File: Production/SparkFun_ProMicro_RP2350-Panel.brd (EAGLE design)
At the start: 92.7 x 87.1 mm, 702 parts, among them J1 QWIIC_RIGHT_ANGLE, J12 USB Female Type C Connector, J13 QWIIC_RIGHT_ANGLE, J16 USB Female Type C Connector, J17 QWIIC_RIGHT_ANGLE, J2 QWIIC_RIGHT_ANGLE, J20 USB Female Type C Connector, J21 QWIIC_RIGHT_ANGLE, J24 USB Female Type C Connector, J5 USB Female Type C Connector, J8 USB Female Type C Connector, J9 QWIIC_RIGHT_ANGLE, U1 RT9080-33GJ5, U10 W25QXX128MBIT, U11 WS2812_2020, U12 RP2350A, U13 RT9080-33GJ5, U14 W25QXX128MBIT, U15 WS2812_2020, U16 RP2350A, U17 RT9080-33GJ5, U18 W25QXX128MBIT, U19 WS2812_2020, U2 RP2350A, U20 RP2350A, U21 RT9080-33GJ5, U22 W25QXX128MBIT, U23 WS2812_2020, U24 RP2350A, U3 WS2812_2020, U4 W25QXX128MBIT, U5 RT9080-33GJ5, U6 W25QXX128MBIT, U7 WS2812_2020, U8 RP2350A, U9 RT9080-33GJ5, Y1 12MHz, Y2 12MHz, Y3 12MHz, Y4 12MHz, Y5 12MHz, Y6 12MHz

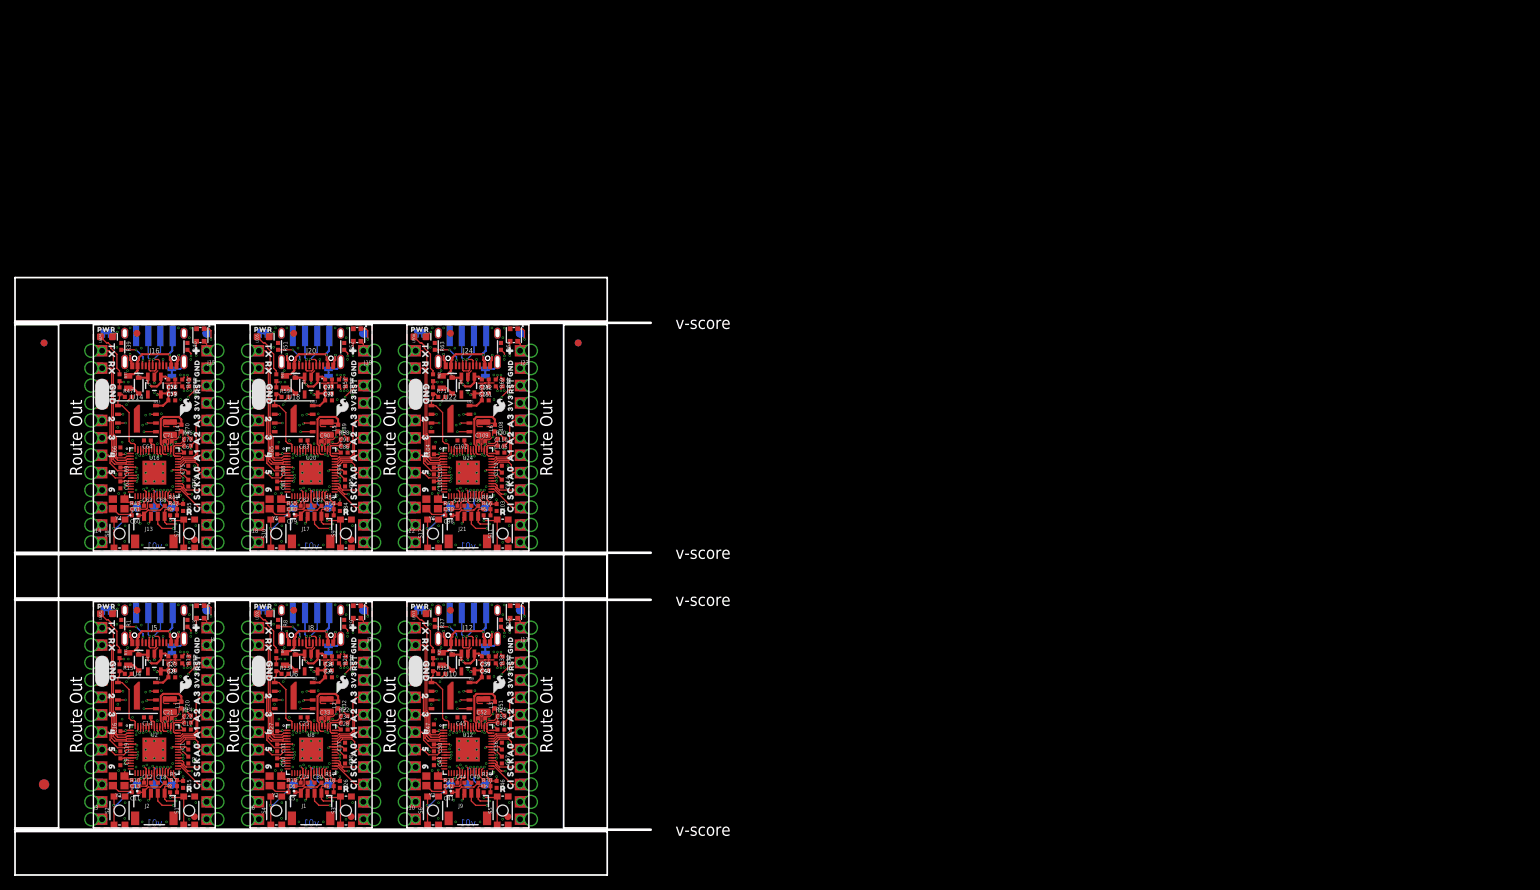
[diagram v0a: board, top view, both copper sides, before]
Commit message: Add v10 production files
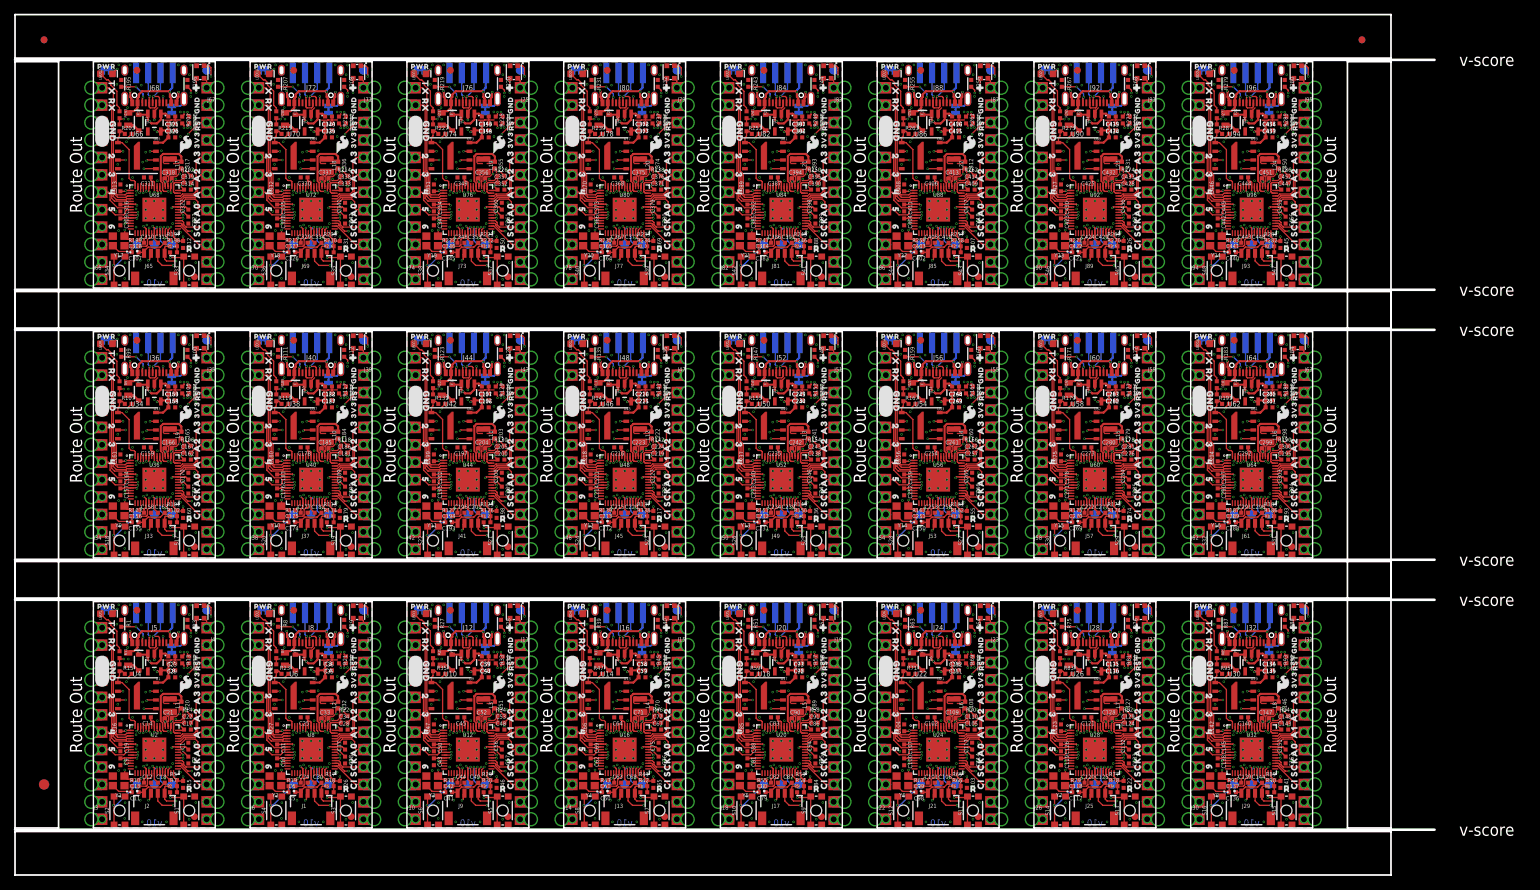
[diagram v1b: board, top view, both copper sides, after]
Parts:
- added C115, C116, C127, C128, C134, C135, C146, C147, C153, C154, C165, C166, C172, C173, C184, C185, C191, C192, C203, C204, C210, C211, C222, C223, C229, C230, C241, C242, C248, C249, C260, C261, C267, C268, C279, C280, C286, C287, C298, C299, C305, C306, C317, C318, C324, C325, C336, C337, C343, C344, C355, C356, C362, C363, C374, C375, C381, C382, C393, C394, C400, C401, C412, C413, C419, C420, C431, C432, C438, C439, C450, C451: 10uF, SparkFun-Capacitors:0402-TIGHT
- added C117, C118, C136, C137, C155, C156, C174, C175, C193, C194, C212, C213, C231, C232, C250, C251, C269, C270, C288, C289, C307, C308, C326, C327, C345, C346, C364, C365, C383, C384, C402, C403, C421, C422, C440, C441: 15pF, SparkFun-Capacitors:0402-TIGHT
- added C119, C120, C121, C122, C123, C124, C125, C126, C130, C132, C133, C138, C139, C140, C141, C142, C143, C144, C145, C149, C151, C152, C157, C158, C159, C160, C161, C162, C163, C164, C168, C170, C171, C176, C177, C178, C179, C180, C181, C182, C183, C187, C189, C190, C195, C196, C197, C198, C199, C200, C201, C202, C206, C208, C209, C214, C215, C216, C217, C218, C219, C220, C221, C225, C227, C228, C233, C234, C235, C236, C237, C238, C239, C240, C244, C246, C247, C252, C253, C254, C255, C256, C257, C258, C259, C263, C265, C266, C271, C272, C273, C274, C275, C276, C277, C278, C282, C284, C285, C290, C291, C292, C293, C294, C295, C296, C297, C301, C303, C304, C309, C310, C311, C312, C313, C314, C315, C316, C320, C322, C323, C328, C329, C330, C331, C332, C333, C334, C335, C339, C341, C342, C347, C348, C349, C350, C351, C352, C353, C354, C358, C360, C361, C366, C367, C368, C369, C370, C371, C372, C373, C377, C379, C380, C385, C386, C387, C388, C389, C390, C391, C392, C396, C398, C399, C404, C405, C406, C407, C408, C409, C410, C411, C415, C417, C418, C423, C424, C425, C426, C427, C428, C429, C430, C434, C436, C437, C442, C443, C444, C445, C446, C447, C448, C449, C453, C455, C456: 0.1uF, SparkFun-Capacitors:0402-TIGHT
- added C129, C131, C148, C150, C167, C169, C186, C188, C205, C207, C224, C226, C243, C245, C262, C264, C281, C283, C300, C302, C319, C321, C338, C340, C357, C359, C376, C378, C395, C397, C414, C416, C433, C435, C452, C454: 2.2uF, SparkFun-Capacitors:0402-TIGHT
- added D10, D11, D12, D13, D14, D15, D16, D17, D18, D19, D20, D21, D22, D23, D24, D7, D8, D9: 3A/10V/280mV, SparkFun-DiscreteSemi:SOD-323
- added F10, F11, F12, F13, F14, F15, F16, F17, F18, F19, F20, F21, F22, F23, F24, F7, F8, F9: 6V 0.5A, SparkFun-Fuses:0805
- added J25, J29, J33, J37, J41, J45, J49, J53, J57, J61, J65, J69, J73, J77, J81, J85, J89, J93: QWIIC_RIGHT_ANGLE, SparkFun-Connectors:JST04_1MM_RA
- added J26, J27, J30, J31, J34, J35, J38, J39, J42, J43, J46, J47, J50, J51, J54, J55, J58, J59, J62, J63, J66, J67, J70, J71, J74, J75, J78, J79, J82, J83, J86, J87, J90, J91, J94, J95: (no value), SparkFun-Connectors:1X12_CASTELLATED
- added J28, J32, J36, J40, J44, J48, J52, J56, J60, J64, J68, J72, J76, J80, J84, J88, J92, J96: USB Female Type C Connector, SparkFun-Connectors:USB-C-16P_4LAYER-PADS
- added JP19, JP20, JP22, JP23, JP25, JP26, JP28, JP29, JP31, JP32, JP34, JP35, JP37, JP38, JP40, JP41, JP43, JP44, JP46, JP47, JP49, JP50, JP52, JP53, JP55, JP56, JP58, JP59, JP61, JP62, JP64, JP65, JP67, JP68, JP70, JP71: FIDUCIAL1X2, SparkFun-Aesthetics:FIDUCIAL-1X2
- added JP21, JP24, JP27, JP30, JP33, JP36, JP39, JP42, JP45, JP48, JP51, JP54, JP57, JP60, JP63, JP66, JP69, JP72: USB_SOLDER_PADS, SparkFun-Connectors:USB-SOLDER-PADS
- added L10, L11, L12, L13, L14, L15, L16, L17, L18, L19, L20, L21, L22, L23, L24, L7, L8, L9: 4.7μH, SparkFun-Coils:1008(2520)
- added LED10, LED11, LED12, LED13, LED14, LED15, LED16, LED17, LED18, LED19, LED20, LED21, LED22, LED23, LED24, LED7, LED8, LED9: Red, SparkFun-LED:LED-0603
- added LOGO19, LOGO22, LOGO25, LOGO28, LOGO31, LOGO34, LOGO37, LOGO40, LOGO43, LOGO46, LOGO49, LOGO52, LOGO55, LOGO58, LOGO61, LOGO64, LOGO67, LOGO70: SFE_LOGO_NAME_FLAME.1_INCH, SparkFun-Aesthetics:SFE_LOGO_NAME_FLAME_.1
- added LOGO20, LOGO23, LOGO26, LOGO29, LOGO32, LOGO35, LOGO38, LOGO41, LOGO44, LOGO47, LOGO50, LOGO53, LOGO56, LOGO59, LOGO62, LOGO65, LOGO68, LOGO71: QWIIC_LOGO_6MM, SparkFun-Aesthetics:QWIIC_6MM
- added LOGO21, LOGO24, LOGO27, LOGO30, LOGO33, LOGO36, LOGO39, LOGO42, LOGO45, LOGO48, LOGO51, LOGO54, LOGO57, LOGO60, LOGO63, LOGO66, LOGO69, LOGO72: SFE_LOGO_FLAME.1_INCH, SparkFun-Aesthetics:SFE_LOGO_FLAME_.1
- added PWR10, PWR11, PWR12, PWR13, PWR14, PWR15, PWR16, PWR17, PWR18, PWR19, PWR20, PWR21, PWR22, PWR23, PWR6, PWR7, PWR8, PWR9, SHLD10, SHLD11, SHLD12, SHLD13, SHLD14, SHLD15, SHLD16, SHLD17, SHLD18, SHLD19, SHLD20, SHLD21, SHLD22, SHLD23, SHLD6, SHLD7, SHLD8, SHLD9: JUMPER-SMT_2_NC_TRACE_SILK, SparkFun-Jumpers:SMT-JUMPER_2_NC_TRACE_SILK
- added R100, R111, R112, R123, R124, R135, R136, R147, R148, R159, R160, R171, R172, R183, R184, R195, R196, R207, R208, R219, R220, R231, R232, R243, R244, R255, R256, R267, R268, R279, R280, R75, R76, R87, R88, R99: 5.1k, SparkFun-Resistors:0402-TIGHT
- added R101, R102, R113, R114, R125, R126, R137, R138, R149, R150, R161, R162, R173, R174, R185, R186, R197, R198, R209, R210, R221, R222, R233, R234, R245, R246, R257, R258, R269, R270, R281, R282, R77, R78, R89, R90: 2.2k, SparkFun-Resistors:0402-TIGHT
- added R103, R107, R115, R119, R127, R131, R139, R143, R151, R155, R163, R167, R175, R179, R187, R191, R199, R203, R211, R215, R223, R227, R235, R239, R247, R251, R259, R263, R271, R275, R283, R287, R79, R83, R91, R95: 1k, SparkFun-Resistors:0402-TIGHT
- added R104, R105, R116, R117, R128, R129, R140, R141, R152, R153, R164, R165, R176, R177, R188, R189, R200, R201, R212, R213, R224, R225, R236, R237, R248, R249, R260, R261, R272, R273, R284, R285, R80, R81, R92, R93: 27, SparkFun-Resistors:0402-TIGHT
- added R106, R118, R130, R142, R154, R166, R178, R190, R202, R214, R226, R238, R250, R262, R274, R286, R82, R94: 10Ω, SparkFun-Resistors:0402-TIGHT
- added R108, R110, R120, R122, R132, R134, R144, R146, R156, R158, R168, R170, R180, R182, R192, R194, R204, R206, R216, R218, R228, R230, R240, R242, R252, R254, R264, R266, R276, R278, R288, R74, R84, R86, R96, R98: 10k, SparkFun-Resistors:0402-TIGHT
- added R109, R121, R133, R145, R157, R169, R181, R193, R205, R217, R229, R241, R253, R265, R277, R73, R85, R97: 4.7k, SparkFun-Resistors:0402-TIGHT
- added S13, S15, S17, S19, S21, S23, S25, S27, S29, S31, S33, S35, S37, S39, S41, S43, S45, S47: Reset, SparkFun-Switches:TACTILE_SWITCH_SMD_4.6X2.8MM
- added S14, S16, S18, S20, S22, S24, S26, S28, S30, S32, S34, S36, S38, S40, S42, S44, S46, S48: Boot, SparkFun-Switches:TACTILE_SWITCH_SMD_4.6X2.8MM
- added TP25, TP26, TP27, TP28, TP29, TP30, TP31, TP32, TP33, TP34, TP35, TP36, TP37, TP38, TP39, TP40, TP41, TP42, TP43, TP44, TP45, TP46, TP47, TP48, TP49, TP50, TP51, TP52, TP53, TP54, TP55, TP56, TP57, TP58, TP59, TP60, TP61, TP62, TP63, TP64, TP65, TP66, TP67, TP68, TP69, TP70, TP71, TP72, TP73, TP74, TP75, TP76, TP77, TP78, TP79, TP80, TP81, TP82, TP83, TP84, TP85, TP86, TP87, TP88, TP89, TP90, TP91, TP92, TP93, TP94, TP95, TP96: TEST-POINT3X5, SparkFun-Connectors:PAD.03X.05
- added U$1000, U$1058, U$1116, U$1174, U$1232, U$1290, U$1348, U$362, U$420, U$478, U$536, U$594, U$652, U$710, U$768, U$826, U$884, U$942: (no value), output:#RST#1
- added U$1001, U$1059, U$1117, U$1175, U$1233, U$1291, U$1349, U$363, U$421, U$479, U$537, U$595, U$653, U$711, U$769, U$827, U$885, U$943: (no value), output:3V30
- added U$1002, U$1060, U$1118, U$1176, U$1234, U$1292, U$1350, U$364, U$422, U$480, U$538, U$596, U$654, U$712, U$770, U$828, U$886, U$944: (no value), output:PWR0
- added U$1003, U$1018, U$1031, U$1061, U$1076, U$1089, U$1119, U$1134, U$1147, U$1177, U$1192, U$1205, U$1235, U$1250, U$1263, U$1293, U$1308, U$1321, U$1351, U$1366, U$1379, U$365, U$380, U$393, U$423, U$438, U$451, U$481, U$496, U$509, U$539, U$554, U$567, U$597, U$612, U$625, U$655, U$670, U$683, U$713, U$728, U$741, U$771, U$786, U$799, U$829, U$844, U$857, U$887, U$902, U$915, U$945, U$960, U$973: (no value), output:GND2
- added U$1004, U$1017, U$1062, U$1075, U$1120, U$1133, U$1178, U$1191, U$1236, U$1249, U$1294, U$1307, U$1352, U$1365, U$366, U$379, U$424, U$437, U$482, U$495, U$540, U$553, U$598, U$611, U$656, U$669, U$714, U$727, U$772, U$785, U$830, U$843, U$888, U$901, U$946, U$959: (no value), output:RX1
- added U$1005, U$1016, U$1063, U$1074, U$1121, U$1132, U$1179, U$1190, U$1237, U$1248, U$1295, U$1306, U$1353, U$1364, U$367, U$378, U$425, U$436, U$483, U$494, U$541, U$552, U$599, U$610, U$657, U$668, U$715, U$726, U$773, U$784, U$831, U$842, U$889, U$900, U$947, U$958: (no value), output:TX0
- added U$1006, U$1064, U$1122, U$1180, U$1238, U$1296, U$1354, U$368, U$426, U$484, U$542, U$600, U$658, U$716, U$774, U$832, U$890, U$948: (no value), output:GND_0
- added U$1007, U$1065, U$1123, U$1181, U$1239, U$1297, U$1355, U$369, U$427, U$485, U$543, U$601, U$659, U$717, U$775, U$833, U$891, U$949: (no value), output:70
- added U$1008, U$1066, U$1124, U$1182, U$1240, U$1298, U$1356, U$370, U$428, U$486, U$544, U$602, U$660, U$718, U$776, U$834, U$892, U$950: (no value), output:81
- added U$1009, U$1067, U$1125, U$1183, U$1241, U$1299, U$1357, U$371, U$429, U$487, U$545, U$603, U$661, U$719, U$777, U$835, U$893, U$951: (no value), output:92
- added U$1010, U$1050, U$1068, U$1108, U$1126, U$1166, U$1184, U$1224, U$1242, U$1282, U$1300, U$1340, U$1358, U$354, U$372, U$412, U$430, U$470, U$488, U$528, U$546, U$586, U$604, U$644, U$662, U$702, U$720, U$760, U$778, U$818, U$836, U$876, U$894, U$934, U$952, U$992: (no value), output:CI4
- added U$1011, U$1052, U$1069, U$1110, U$1127, U$1168, U$1185, U$1226, U$1243, U$1284, U$1301, U$1342, U$1359, U$356, U$373, U$414, U$431, U$472, U$489, U$530, U$547, U$588, U$605, U$646, U$663, U$704, U$721, U$762, U$779, U$820, U$837, U$878, U$895, U$936, U$953, U$994: (no value), output:SCK3
- added U$1012, U$1046, U$1070, U$1104, U$1128, U$1162, U$1186, U$1220, U$1244, U$1278, U$1302, U$1336, U$1360, U$350, U$374, U$408, U$432, U$466, U$490, U$524, U$548, U$582, U$606, U$640, U$664, U$698, U$722, U$756, U$780, U$814, U$838, U$872, U$896, U$930, U$954, U$988: (no value), output:A00
- added U$1013, U$1047, U$1071, U$1105, U$1129, U$1163, U$1187, U$1221, U$1245, U$1279, U$1303, U$1337, U$1361, U$351, U$375, U$409, U$433, U$467, U$491, U$525, U$549, U$583, U$607, U$641, U$665, U$699, U$723, U$757, U$781, U$815, U$839, U$873, U$897, U$931, U$955, U$989: (no value), output:A10
- added U$1014, U$1048, U$1072, U$1106, U$1130, U$1164, U$1188, U$1222, U$1246, U$1280, U$1304, U$1338, U$1362, U$352, U$376, U$410, U$434, U$468, U$492, U$526, U$550, U$584, U$608, U$642, U$666, U$700, U$724, U$758, U$782, U$816, U$840, U$874, U$898, U$932, U$956, U$990: (no value), output:A21
- added U$1015, U$1049, U$1073, U$1107, U$1131, U$1165, U$1189, U$1223, U$1247, U$1281, U$1305, U$1339, U$1363, U$353, U$377, U$411, U$435, U$469, U$493, U$527, U$551, U$585, U$609, U$643, U$667, U$701, U$725, U$759, U$783, U$817, U$841, U$875, U$899, U$933, U$957, U$991: (no value), output:A32
- added U$1019, U$1053, U$1077, U$1111, U$1135, U$1169, U$1193, U$1227, U$1251, U$1285, U$1309, U$1343, U$1367, U$357, U$381, U$415, U$439, U$473, U$497, U$531, U$555, U$589, U$613, U$647, U$671, U$705, U$729, U$763, U$787, U$821, U$845, U$879, U$903, U$937, U$961, U$995: (no value), output:20
- added U$1020, U$1054, U$1078, U$1112, U$1136, U$1170, U$1194, U$1228, U$1252, U$1286, U$1310, U$1344, U$1368, U$358, U$382, U$416, U$440, U$474, U$498, U$532, U$556, U$590, U$614, U$648, U$672, U$706, U$730, U$764, U$788, U$822, U$846, U$880, U$904, U$938, U$962, U$996: (no value), output:31
- added U$1021, U$1055, U$1079, U$1113, U$1137, U$1171, U$1195, U$1229, U$1253, U$1287, U$1311, U$1345, U$1369, U$359, U$383, U$417, U$441, U$475, U$499, U$533, U$557, U$591, U$615, U$649, U$673, U$707, U$731, U$765, U$789, U$823, U$847, U$881, U$905, U$939, U$963, U$997: (no value), output:42
- added U$1022, U$1056, U$1080, U$1114, U$1138, U$1172, U$1196, U$1230, U$1254, U$1288, U$1312, U$1346, U$1370, U$360, U$384, U$418, U$442, U$476, U$500, U$534, U$558, U$592, U$616, U$650, U$674, U$708, U$732, U$766, U$790, U$824, U$848, U$882, U$906, U$940, U$964, U$998: (no value), output:53
- added U$1023, U$1057, U$1081, U$1115, U$1139, U$1173, U$1197, U$1231, U$1255, U$1289, U$1313, U$1347, U$1371, U$361, U$385, U$419, U$443, U$477, U$501, U$535, U$559, U$593, U$617, U$651, U$675, U$709, U$733, U$767, U$791, U$825, U$849, U$883, U$907, U$941, U$965, U$999: (no value), output:64
- added U$1024, U$1082, U$1140, U$1198, U$1256, U$1314, U$1372, U$386, U$444, U$502, U$560, U$618, U$676, U$734, U$792, U$850, U$908, U$966: (no value), output:D#1
- added U$1025, U$1083, U$1141, U$1199, U$1257, U$1315, U$1373, U$387, U$445, U$503, U$561, U$619, U$677, U$735, U$793, U$851, U$909, U$967: (no value), output:D#2
- added U$1026, U$1084, U$1142, U$1200, U$1258, U$1316, U$1374, U$388, U$446, U$504, U$562, U$620, U$678, U$736, U$794, U$852, U$910, U$968: (no value), output:G0
- added U$1027, U$1085, U$1143, U$1201, U$1259, U$1317, U$1375, U$389, U$447, U$505, U$563, U$621, U$679, U$737, U$795, U$853, U$911, U$969: (no value), output:V3
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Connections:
- new net !RESET!10: J43.3, J43.3B, R122.1, S21.3, S21.4, U44.26
- new net !RESET!11: J47.3, J47.3B, R134.1, S23.3, S23.4, U48.26
- new net !RESET!12: J51.3, J51.3B, R146.1, S25.3, S25.4, U52.26
- new net !RESET!13: J55.3, J55.3B, R158.1, S27.3, S27.4, U56.26
- new net !RESET!14: J59.3, J59.3B, R170.1, S29.3, S29.4, U60.26
- new net !RESET!15: J63.3, J63.3B, R182.1, S31.3, S31.4, U64.26
- new net !RESET!16: J67.3, J67.3B, R194.1, S33.3, S33.4, U68.26
- new net !RESET!17: J71.3, J71.3B, R206.1, S35.3, S35.4, U72.26
- new net !RESET!18: J75.3, J75.3B, R218.1, S37.3, S37.4, U76.26
- new net !RESET!19: J79.3, J79.3B, R230.1, S39.3, S39.4, U80.26
- new net !RESET!20: J83.3, J83.3B, R242.1, S41.3, S41.4, U84.26
- new net !RESET!21: J87.3, J87.3B, R254.1, S43.3, S43.4, U88.26
- new net !RESET!22: J91.3, J91.3B, R266.1, S45.3, S45.4, U92.26
- new net !RESET!23: J95.3, J95.3B, R278.1, S47.3, S47.4, U96.26
- new net !RESET!6: J27.3, J27.3B, R74.1, S13.3, S13.4, U28.26
- new net !RESET!7: J31.3, J31.3B, R86.1, S15.3, S15.4, U32.26
- new net !RESET!8: J35.3, J35.3B, R98.1, S17.3, S17.4, U36.26
- new net !RESET!9: J39.3, J39.3B, R110.1, S19.3, S19.4, U40.26
- new net 0/TX10: J42.12, J42.12B, U44.2
- new net 0/TX11: J46.12, J46.12B, U48.2
- new net 0/TX12: J50.12, J50.12B, U52.2
- new net 0/TX13: J54.12, J54.12B, U56.2
- new net 0/TX14: J58.12, J58.12B, U60.2
- new net 0/TX15: J62.12, J62.12B, U64.2
- new net 0/TX16: J66.12, J66.12B, U68.2
- new net 0/TX17: J70.12, J70.12B, U72.2
- new net 0/TX18: J74.12, J74.12B, U76.2
- new net 0/TX19: J78.12, J78.12B, U80.2
- new net 0/TX20: J82.12, J82.12B, U84.2
- new net 0/TX21: J86.12, J86.12B, U88.2
- new net 0/TX22: J90.12, J90.12B, U92.2
- new net 0/TX23: J94.12, J94.12B, U96.2
- new net 0/TX6: J26.12, J26.12B, U28.2
- new net 0/TX7: J30.12, J30.12B, U32.2
- new net 0/TX8: J34.12, J34.12B, U36.2
- new net 0/TX9: J38.12, J38.12B, U40.2
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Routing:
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- added copper zone on layer 1, net 1.1V10
- added copper zone on layer 1, net 1.1V11
- added copper zone on layer 1, net 1.1V12
- added copper zone on layer 1, net 1.1V13
- added copper zone on layer 1, net 1.1V14
- added copper zone on layer 1, net 1.1V15
- added copper zone on layer 1, net 1.1V16
- added copper zone on layer 1, net 1.1V17
- added copper zone on layer 1, net 1.1V18
- added copper zone on layer 1, net 1.1V19
- added copper zone on layer 1, net 1.1V20
- added copper zone on layer 1, net 1.1V21
- added copper zone on layer 1, net 1.1V22
- added copper zone on layer 1, net 1.1V23
- added copper zone on layer 1, net 1.1V6
- added copper zone on layer 1, net 1.1V7
- added copper zone on layer 1, net 1.1V8
- added copper zone on layer 1, net 1.1V9
- added copper zone on layer 1, net 3.3V10
- added copper zone on layer 15, net 3.3V10
- added copper zone on layer 1, net 3.3V11
- added copper zone on layer 15, net 3.3V11
- added copper zone on layer 1, net 3.3V12
- added copper zone on layer 15, net 3.3V12
- added copper zone on layer 1, net 3.3V13
- added copper zone on layer 15, net 3.3V13
- added copper zone on layer 1, net 3.3V14
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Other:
- board size 92.7 x 87.1 mm -> 207 x 125.5 mm
- board text added: "v10"
- board text removed: "v01"

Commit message: Add v09 panel files
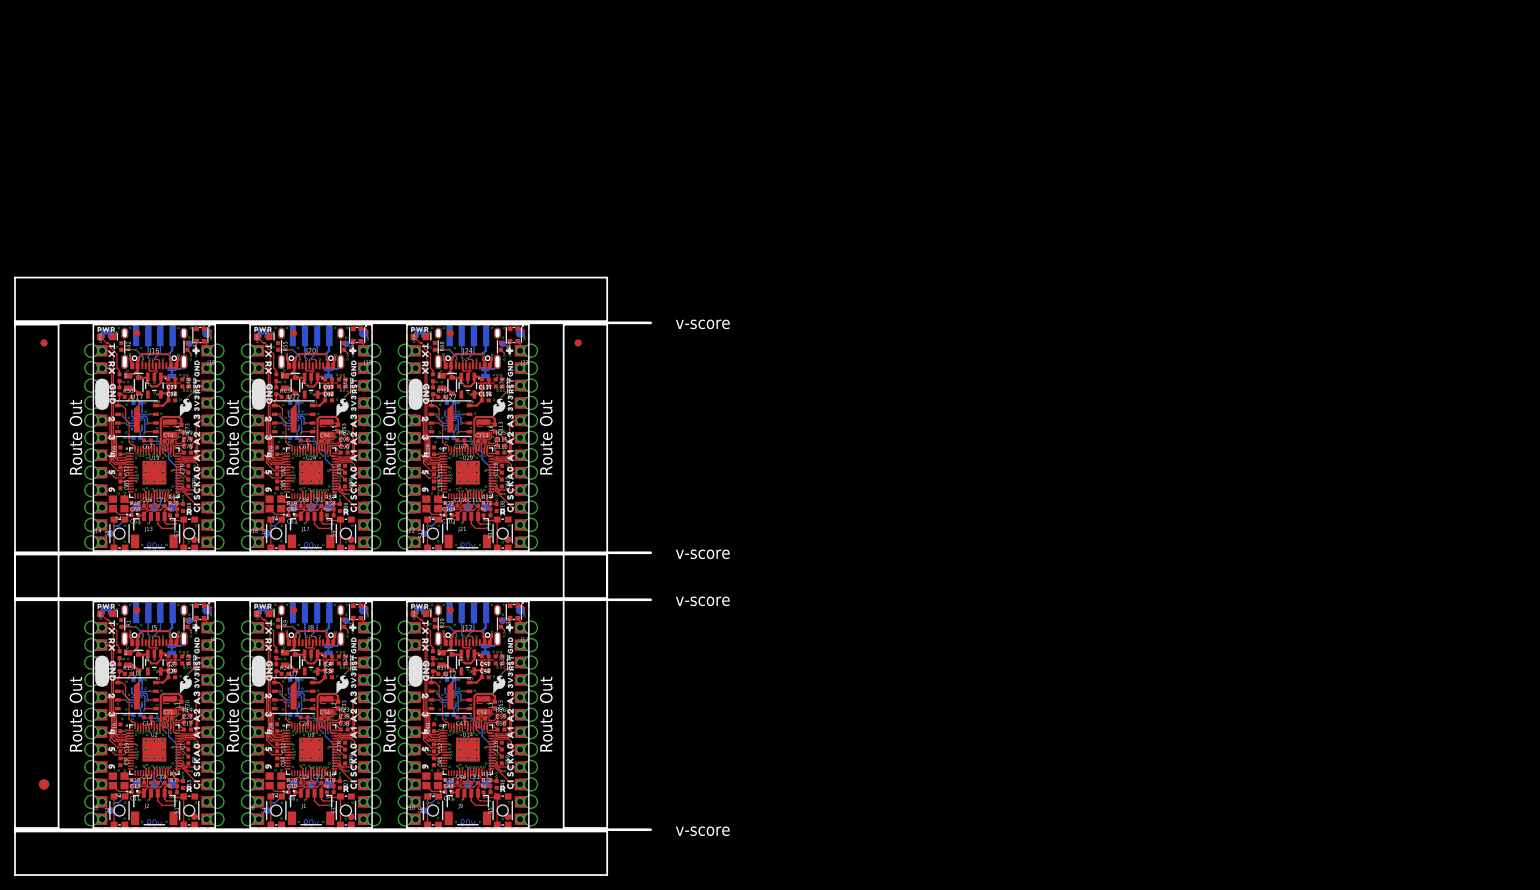
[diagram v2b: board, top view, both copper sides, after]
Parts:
- removed C121, C122, C123, C124, C125, C126, C130, C132, C133, C138, C139, C140, C141, C142, C143, C144, C145, C149, C151, C152, C157, C158, C159, C160, C161, C162, C163, C164, C168, C170, C171, C176, C177, C178, C179, C180, C181, C182, C183, C187, C189, C190, C195, C196, C197, C198, C199, C200, C201, C202, C206, C208, C209, C214, C215, C216, C217, C218, C219, C220, C221, C225, C227, C228, C233, C234, C235, C236, C237, C238, C239, C240, C244, C246, C247, C252, C253, C254, C255, C256, C257, C258, C259, C263, C265, C266, C271, C272, C273, C274, C275, C276, C277, C278, C282, C284, C285, C290, C291, C292, C293, C294, C295, C296, C297, C301, C303, C304, C309, C310, C311, C312, C313, C314, C315, C316, C320, C322, C323, C328, C329, C330, C331, C332, C333, C334, C335, C339, C341, C342, C347, C348, C349, C350, C351, C352, C353, C354, C358, C360, C361, C366, C367, C368, C369, C370, C371, C372, C373, C377, C379, C380, C385, C386, C387, C388, C389, C390, C391, C392, C396, C398, C399, C404, C405, C406, C407, C408, C409, C410, C411, C415, C417, C418, C423, C424, C425, C426, C427, C428, C429, C430, C434, C436, C437, C442, C443, C444, C445, C446, C447, C448, C449, C453, C455, C456: 0.1uF, SparkFun-Capacitors:0402-TIGHT
- removed C127, C128, C134, C135, C146, C147, C153, C154, C165, C166, C172, C173, C184, C185, C191, C192, C203, C204, C210, C211, C222, C223, C229, C230, C241, C242, C248, C249, C260, C261, C267, C268, C279, C280, C286, C287, C298, C299, C305, C306, C317, C318, C324, C325, C336, C337, C343, C344, C355, C356, C362, C363, C374, C375, C381, C382, C393, C394, C400, C401, C412, C413, C419, C420, C431, C432, C438, C439, C450, C451: 10uF, SparkFun-Capacitors:0402-TIGHT
- removed C129, C131, C148, C150, C167, C169, C186, C188, C205, C207, C224, C226, C243, C245, C262, C264, C281, C283, C300, C302, C319, C321, C338, C340, C357, C359, C376, C378, C395, C397, C414, C416, C433, C435, C452, C454: 2.2uF, SparkFun-Capacitors:0402-TIGHT
- removed C136, C137, C155, C156, C174, C175, C193, C194, C212, C213, C231, C232, C250, C251, C269, C270, C288, C289, C307, C308, C326, C327, C345, C346, C364, C365, C383, C384, C402, C403, C421, C422, C440, C441: 15pF, SparkFun-Capacitors:0402-TIGHT
- removed D10, D11, D12, D13, D14, D15, D16, D17, D18, D19, D20, D21, D22, D23, D24, D7, D8, D9: 3A/10V/280mV, SparkFun-DiscreteSemi:SOD-323
- removed F10, F11, F12, F13, F14, F15, F16, F17, F18, F19, F20, F21, F22, F23, F24, F7, F8, F9: 6V 0.5A, SparkFun-Fuses:0805
- removed J25, J29, J33, J37, J41, J45, J49, J53, J57, J61, J65, J69, J73, J77, J81, J85, J89, J93: QWIIC_RIGHT_ANGLE, SparkFun-Connectors:JST04_1MM_RA
- removed J26, J27, J30, J31, J34, J35, J38, J39, J42, J43, J46, J47, J50, J51, J54, J55, J58, J59, J62, J63, J66, J67, J70, J71, J74, J75, J78, J79, J82, J83, J86, J87, J90, J91, J94, J95: (no value), SparkFun-Connectors:1X12_CASTELLATED
- removed J28, J32, J36, J40, J44, J48, J52, J56, J60, J64, J68, J72, J76, J80, J84, J88, J92, J96: USB Female Type C Connector, SparkFun-Connectors:USB-C-16P_4LAYER-PADS
- removed JP31, JP32, JP34, JP35, JP37, JP38, JP40, JP41, JP43, JP44, JP46, JP47, JP49, JP50, JP52, JP53, JP55, JP56, JP58, JP59, JP61, JP62, JP64, JP65, JP67, JP68, JP70, JP71: FIDUCIAL1X2, SparkFun-Aesthetics:FIDUCIAL-1X2
- removed JP33, JP36, JP39, JP42, JP45, JP48, JP51, JP54, JP57, JP60, JP63, JP66, JP69, JP72: USB_SOLDER_PADS, SparkFun-Connectors:USB-SOLDER-PADS
- removed L10, L11, L12, L13, L14, L15, L16, L17, L18, L19, L20, L21, L22, L23, L24, L7, L8, L9: 4.7μH, SparkFun-Coils:1008(2520)
- removed LED10, LED11, LED12, LED13, LED14, LED15, LED16, LED17, LED18, LED19, LED20, LED21, LED22, LED23, LED24, LED7, LED8, LED9: Red, SparkFun-LED:LED-0603
- removed LOGO19, LOGO22, LOGO25, LOGO28, LOGO31, LOGO34, LOGO37, LOGO40, LOGO43, LOGO46, LOGO49, LOGO52, LOGO55, LOGO58, LOGO61, LOGO64, LOGO67, LOGO70: SFE_LOGO_NAME_FLAME.1_INCH, SparkFun-Aesthetics:SFE_LOGO_NAME_FLAME_.1
- removed LOGO20, LOGO23, LOGO26, LOGO29, LOGO32, LOGO35, LOGO38, LOGO41, LOGO44, LOGO47, LOGO50, LOGO53, LOGO56, LOGO59, LOGO62, LOGO65, LOGO68, LOGO71: QWIIC_LOGO_6MM, SparkFun-Aesthetics:QWIIC_6MM
- removed LOGO21, LOGO24, LOGO27, LOGO30, LOGO33, LOGO36, LOGO39, LOGO42, LOGO45, LOGO48, LOGO51, LOGO54, LOGO57, LOGO60, LOGO63, LOGO66, LOGO69, LOGO72: SFE_LOGO_FLAME.1_INCH, SparkFun-Aesthetics:SFE_LOGO_FLAME_.1
- removed PWR10, PWR11, PWR12, PWR13, PWR14, PWR15, PWR16, PWR17, PWR18, PWR19, PWR20, PWR21, PWR22, PWR23, PWR6, PWR7, PWR8, PWR9, SHLD10, SHLD11, SHLD12, SHLD13, SHLD14, SHLD15, SHLD16, SHLD17, SHLD18, SHLD19, SHLD20, SHLD21, SHLD22, SHLD23, SHLD6, SHLD7, SHLD8, SHLD9: JUMPER-SMT_2_NC_TRACE_SILK, SparkFun-Jumpers:SMT-JUMPER_2_NC_TRACE_SILK
- removed R100, R111, R112, R123, R124, R135, R136, R147, R148, R159, R160, R171, R172, R183, R184, R195, R196, R207, R208, R219, R220, R231, R232, R243, R244, R255, R256, R267, R268, R279, R280, R87, R88, R99: 5.1k, SparkFun-Resistors:0402-TIGHT
- removed R101, R102, R113, R114, R125, R126, R137, R138, R149, R150, R161, R162, R173, R174, R185, R186, R197, R198, R209, R210, R221, R222, R233, R234, R245, R246, R257, R258, R269, R270, R281, R282, R89, R90: 2.2k, SparkFun-Resistors:0402-TIGHT
- removed R103, R107, R115, R119, R127, R131, R139, R143, R151, R155, R163, R167, R175, R179, R187, R191, R199, R203, R211, R215, R223, R227, R235, R239, R247, R251, R259, R263, R271, R275, R283, R287, R79, R83, R91, R95: 1k, SparkFun-Resistors:0402-TIGHT
- removed R104, R105, R116, R117, R128, R129, R140, R141, R152, R153, R164, R165, R176, R177, R188, R189, R200, R201, R212, R213, R224, R225, R236, R237, R248, R249, R260, R261, R272, R273, R284, R285, R80, R81, R92, R93: 27, SparkFun-Resistors:0402-TIGHT
- removed R106, R118, R130, R142, R154, R166, R178, R190, R202, R214, R226, R238, R250, R262, R274, R286, R82, R94: 10Ω, SparkFun-Resistors:0402-TIGHT
- removed R108, R110, R120, R122, R132, R134, R144, R146, R156, R158, R168, R170, R180, R182, R192, R194, R204, R206, R216, R218, R228, R230, R240, R242, R252, R254, R264, R266, R276, R278, R288, R84, R86, R96, R98: 10k, SparkFun-Resistors:0402-TIGHT
- removed R109, R121, R133, R145, R157, R169, R181, R193, R205, R217, R229, R241, R253, R265, R277, R85, R97: 4.7k, SparkFun-Resistors:0402-TIGHT
- removed S13, S15, S17, S19, S21, S23, S25, S27, S29, S31, S33, S35, S37, S39, S41, S43, S45, S47: Reset, SparkFun-Switches:TACTILE_SWITCH_SMD_4.6X2.8MM
- removed S14, S16, S18, S20, S22, S24, S26, S28, S30, S32, S34, S36, S38, S40, S42, S44, S46, S48: Boot, SparkFun-Switches:TACTILE_SWITCH_SMD_4.6X2.8MM
- removed TP25, TP26, TP27, TP28, TP29, TP30, TP31, TP32, TP33, TP34, TP35, TP36, TP37, TP38, TP39, TP40, TP41, TP42, TP43, TP44, TP45, TP46, TP47, TP48, TP49, TP50, TP51, TP52, TP53, TP54, TP55, TP56, TP57, TP58, TP59, TP60, TP61, TP62, TP63, TP64, TP65, TP66, TP67, TP68, TP69, TP70, TP71, TP72, TP73, TP74, TP75, TP76, TP77, TP78, TP79, TP80, TP81, TP82, TP83, TP84, TP85, TP86, TP87, TP88, TP89, TP90, TP91, TP92, TP93, TP94, TP95, TP96: TEST-POINT3X5, SparkFun-Connectors:PAD.03X.05
- removed U$1000, U$1058, U$1116, U$1174, U$1232, U$1290, U$1348, U$362, U$420, U$478, U$536, U$594, U$652, U$710, U$768, U$826, U$884, U$942: (no value), output:#RST#1
- removed U$1001, U$1059, U$1117, U$1175, U$1233, U$1291, U$1349, U$363, U$421, U$479, U$537, U$595, U$653, U$711, U$769, U$827, U$885, U$943: (no value), output:3V30
- removed U$1002, U$1060, U$1118, U$1176, U$1234, U$1292, U$1350, U$364, U$422, U$480, U$538, U$596, U$654, U$712, U$770, U$828, U$886, U$944: (no value), output:PWR0
- removed U$1003, U$1018, U$1031, U$1061, U$1076, U$1089, U$1119, U$1134, U$1147, U$1177, U$1192, U$1205, U$1235, U$1250, U$1263, U$1293, U$1308, U$1321, U$1351, U$1366, U$1379, U$365, U$380, U$393, U$423, U$438, U$451, U$481, U$496, U$509, U$539, U$554, U$567, U$597, U$612, U$625, U$655, U$670, U$683, U$713, U$728, U$741, U$771, U$786, U$799, U$829, U$844, U$857, U$887, U$902, U$915, U$945, U$960, U$973: (no value), output:GND2
- removed U$1004, U$1017, U$1062, U$1075, U$1120, U$1133, U$1178, U$1191, U$1236, U$1249, U$1294, U$1307, U$1352, U$1365, U$366, U$379, U$424, U$437, U$482, U$495, U$540, U$553, U$598, U$611, U$656, U$669, U$714, U$727, U$772, U$785, U$830, U$843, U$888, U$901, U$946, U$959: (no value), output:RX1
- removed U$1005, U$1016, U$1063, U$1074, U$1121, U$1132, U$1179, U$1190, U$1237, U$1248, U$1295, U$1306, U$1353, U$1364, U$367, U$378, U$425, U$436, U$483, U$494, U$541, U$552, U$599, U$610, U$657, U$668, U$715, U$726, U$773, U$784, U$831, U$842, U$889, U$900, U$947, U$958: (no value), output:TX0
- removed U$1006, U$1064, U$1122, U$1180, U$1238, U$1296, U$1354, U$368, U$426, U$484, U$542, U$600, U$658, U$716, U$774, U$832, U$890, U$948: (no value), output:GND_0
- removed U$1007, U$1065, U$1123, U$1181, U$1239, U$1297, U$1355, U$369, U$427, U$485, U$543, U$601, U$659, U$717, U$775, U$833, U$891, U$949: (no value), output:70
- removed U$1008, U$1066, U$1124, U$1182, U$1240, U$1298, U$1356, U$370, U$428, U$486, U$544, U$602, U$660, U$718, U$776, U$834, U$892, U$950: (no value), output:81
- removed U$1009, U$1067, U$1125, U$1183, U$1241, U$1299, U$1357, U$371, U$429, U$487, U$545, U$603, U$661, U$719, U$777, U$835, U$893, U$951: (no value), output:92
- removed U$1010, U$1050, U$1068, U$1108, U$1126, U$1166, U$1184, U$1224, U$1242, U$1282, U$1300, U$1340, U$1358, U$354, U$372, U$412, U$430, U$470, U$488, U$528, U$546, U$586, U$604, U$644, U$662, U$702, U$720, U$760, U$778, U$818, U$836, U$876, U$894, U$934, U$952, U$992: (no value), output:CI4
- removed U$1011, U$1052, U$1069, U$1110, U$1127, U$1168, U$1185, U$1226, U$1243, U$1284, U$1301, U$1342, U$1359, U$356, U$373, U$414, U$431, U$472, U$489, U$530, U$547, U$588, U$605, U$646, U$663, U$704, U$721, U$762, U$779, U$820, U$837, U$878, U$895, U$936, U$953, U$994: (no value), output:SCK3
- removed U$1012, U$1046, U$1070, U$1104, U$1128, U$1162, U$1186, U$1220, U$1244, U$1278, U$1302, U$1336, U$1360, U$350, U$374, U$408, U$432, U$466, U$490, U$524, U$548, U$582, U$606, U$640, U$664, U$698, U$722, U$756, U$780, U$814, U$838, U$872, U$896, U$930, U$954, U$988: (no value), output:A00
- removed U$1013, U$1047, U$1071, U$1105, U$1129, U$1163, U$1187, U$1221, U$1245, U$1279, U$1303, U$1337, U$1361, U$351, U$375, U$409, U$433, U$467, U$491, U$525, U$549, U$583, U$607, U$641, U$665, U$699, U$723, U$757, U$781, U$815, U$839, U$873, U$897, U$931, U$955, U$989: (no value), output:A10
- removed U$1014, U$1048, U$1072, U$1106, U$1130, U$1164, U$1188, U$1222, U$1246, U$1280, U$1304, U$1338, U$1362, U$352, U$376, U$410, U$434, U$468, U$492, U$526, U$550, U$584, U$608, U$642, U$666, U$700, U$724, U$758, U$782, U$816, U$840, U$874, U$898, U$932, U$956, U$990: (no value), output:A21
- removed U$1015, U$1049, U$1073, U$1107, U$1131, U$1165, U$1189, U$1223, U$1247, U$1281, U$1305, U$1339, U$1363, U$353, U$377, U$411, U$435, U$469, U$493, U$527, U$551, U$585, U$609, U$643, U$667, U$701, U$725, U$759, U$783, U$817, U$841, U$875, U$899, U$933, U$957, U$991: (no value), output:A32
- removed U$1019, U$1053, U$1077, U$1111, U$1135, U$1169, U$1193, U$1227, U$1251, U$1285, U$1309, U$1343, U$1367, U$357, U$381, U$415, U$439, U$473, U$497, U$531, U$555, U$589, U$613, U$647, U$671, U$705, U$729, U$763, U$787, U$821, U$845, U$879, U$903, U$937, U$961, U$995: (no value), output:20
- removed U$1020, U$1054, U$1078, U$1112, U$1136, U$1170, U$1194, U$1228, U$1252, U$1286, U$1310, U$1344, U$1368, U$358, U$382, U$416, U$440, U$474, U$498, U$532, U$556, U$590, U$614, U$648, U$672, U$706, U$730, U$764, U$788, U$822, U$846, U$880, U$904, U$938, U$962, U$996: (no value), output:31
- removed U$1021, U$1055, U$1079, U$1113, U$1137, U$1171, U$1195, U$1229, U$1253, U$1287, U$1311, U$1345, U$1369, U$359, U$383, U$417, U$441, U$475, U$499, U$533, U$557, U$591, U$615, U$649, U$673, U$707, U$731, U$765, U$789, U$823, U$847, U$881, U$905, U$939, U$963, U$997: (no value), output:42
- removed U$1022, U$1056, U$1080, U$1114, U$1138, U$1172, U$1196, U$1230, U$1254, U$1288, U$1312, U$1346, U$1370, U$360, U$384, U$418, U$442, U$476, U$500, U$534, U$558, U$592, U$616, U$650, U$674, U$708, U$732, U$766, U$790, U$824, U$848, U$882, U$906, U$940, U$964, U$998: (no value), output:53
- removed U$1023, U$1057, U$1081, U$1115, U$1139, U$1173, U$1197, U$1231, U$1255, U$1289, U$1313, U$1347, U$1371, U$361, U$385, U$419, U$443, U$477, U$501, U$535, U$559, U$593, U$617, U$651, U$675, U$709, U$733, U$767, U$791, U$825, U$849, U$883, U$907, U$941, U$965, U$999: (no value), output:64
- removed U$1024, U$1082, U$1140, U$1198, U$1256, U$1314, U$1372, U$386, U$444, U$502, U$560, U$618, U$676, U$734, U$792, U$850, U$908, U$966: (no value), output:D#1
- removed U$1025, U$1083, U$1141, U$1199, U$1257, U$1315, U$1373, U$387, U$445, U$503, U$561, U$619, U$677, U$735, U$793, U$851, U$909, U$967: (no value), output:D#2
- removed U$1026, U$1084, U$1142, U$1200, U$1258, U$1316, U$1374, U$388, U$446, U$504, U$562, U$620, U$678, U$736, U$794, U$852, U$910, U$968: (no value), output:G0
- removed U$1027, U$1085, U$1143, U$1201, U$1259, U$1317, U$1375, U$389, U$447, U$505, U$563, U$621, U$679, U$737, U$795, U$853, U$911, U$969: (no value), output:V3
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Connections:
- net QSPI-CS renamed FLASH_!CS!/BOOT
- removed net !RESET!10: J43.3, J43.3B, R122.1, S21.3, S21.4, U44.26
- removed net !RESET!11: J47.3, J47.3B, R134.1, S23.3, S23.4, U48.26
- removed net !RESET!12: J51.3, J51.3B, R146.1, S25.3, S25.4, U52.26
- removed net !RESET!13: J55.3, J55.3B, R158.1, S27.3, S27.4, U56.26
- removed net !RESET!14: J59.3, J59.3B, R170.1, S29.3, S29.4, U60.26
- removed net !RESET!15: J63.3, J63.3B, R182.1, S31.3, S31.4, U64.26
- removed net !RESET!16: J67.3, J67.3B, R194.1, S33.3, S33.4, U68.26
- removed net !RESET!17: J71.3, J71.3B, R206.1, S35.3, S35.4, U72.26
- removed net !RESET!18: J75.3, J75.3B, R218.1, S37.3, S37.4, U76.26
- removed net !RESET!19: J79.3, J79.3B, R230.1, S39.3, S39.4, U80.26
- removed net !RESET!20: J83.3, J83.3B, R242.1, S41.3, S41.4, U84.26
- removed net !RESET!21: J87.3, J87.3B, R254.1, S43.3, S43.4, U88.26
- removed net !RESET!22: J91.3, J91.3B, R266.1, S45.3, S45.4, U92.26
- removed net !RESET!23: J95.3, J95.3B, R278.1, S47.3, S47.4, U96.26
- removed net !RESET!6: J27.3, J27.3B, R74.1, S13.3, S13.4, U28.26
- removed net !RESET!7: J31.3, J31.3B, R86.1, S15.3, S15.4, U32.26
- removed net !RESET!8: J35.3, J35.3B, R98.1, S17.3, S17.4, U36.26
- removed net !RESET!9: J39.3, J39.3B, R110.1, S19.3, S19.4, U40.26
- removed net 0/TX10: J42.12, J42.12B, U44.2
- removed net 0/TX11: J46.12, J46.12B, U48.2
- removed net 0/TX12: J50.12, J50.12B, U52.2
- removed net 0/TX13: J54.12, J54.12B, U56.2
- removed net 0/TX14: J58.12, J58.12B, U60.2
- removed net 0/TX15: J62.12, J62.12B, U64.2
- removed net 0/TX16: J66.12, J66.12B, U68.2
- removed net 0/TX17: J70.12, J70.12B, U72.2
- removed net 0/TX18: J74.12, J74.12B, U76.2
- removed net 0/TX19: J78.12, J78.12B, U80.2
- removed net 0/TX20: J82.12, J82.12B, U84.2
- removed net 0/TX21: J86.12, J86.12B, U88.2
- removed net 0/TX22: J90.12, J90.12B, U92.2
- removed net 0/TX23: J94.12, J94.12B, U96.2
- removed net 0/TX6: J26.12, J26.12B, U28.2
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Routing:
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- removed copper zone on layer 1, net 1.1V10
- removed copper zone on layer 1, net 1.1V11
- removed copper zone on layer 1, net 1.1V12
- removed copper zone on layer 1, net 1.1V13
- removed copper zone on layer 1, net 1.1V14
- removed copper zone on layer 1, net 1.1V15
- removed copper zone on layer 1, net 1.1V16
- removed copper zone on layer 1, net 1.1V17
- removed copper zone on layer 1, net 1.1V18
- removed copper zone on layer 1, net 1.1V19
- removed copper zone on layer 1, net 1.1V20
- removed copper zone on layer 1, net 1.1V21
- removed copper zone on layer 1, net 1.1V22
- removed copper zone on layer 1, net 1.1V23
- removed copper zone on layer 1, net 1.1V6
- removed copper zone on layer 1, net 1.1V7
- removed copper zone on layer 1, net 1.1V8
- removed copper zone on layer 1, net 1.1V9
- removed copper zone on layer 1, net 3.3V10
- removed copper zone on layer 15, net 3.3V10
- removed copper zone on layer 1, net 3.3V11
- removed copper zone on layer 15, net 3.3V11
- removed copper zone on layer 1, net 3.3V12
- removed copper zone on layer 15, net 3.3V12
- removed copper zone on layer 1, net 3.3V13
- removed copper zone on layer 15, net 3.3V13
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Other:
- board size 207 x 125.5 mm -> 92.7 x 87.1 mm
- board text added: "v09"
- board text removed: "v10"
